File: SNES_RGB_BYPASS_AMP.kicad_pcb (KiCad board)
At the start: 2 copper layers, 16 x 29.5 mm, 16 parts, among them J1 RGB_Input, J2 SNES Multiout, U1 THS7374

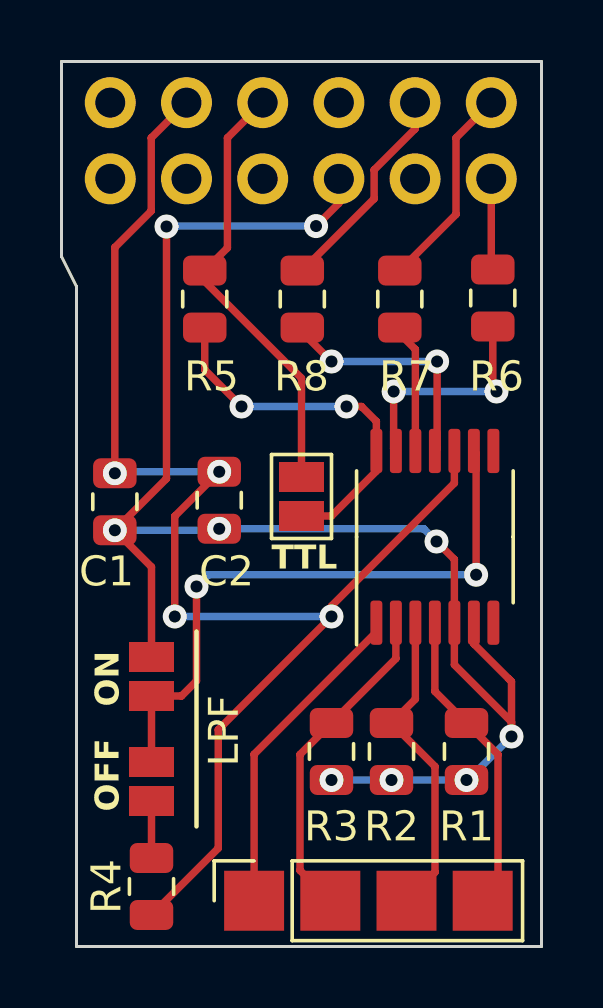
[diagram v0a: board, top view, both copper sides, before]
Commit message: Update silkscreen
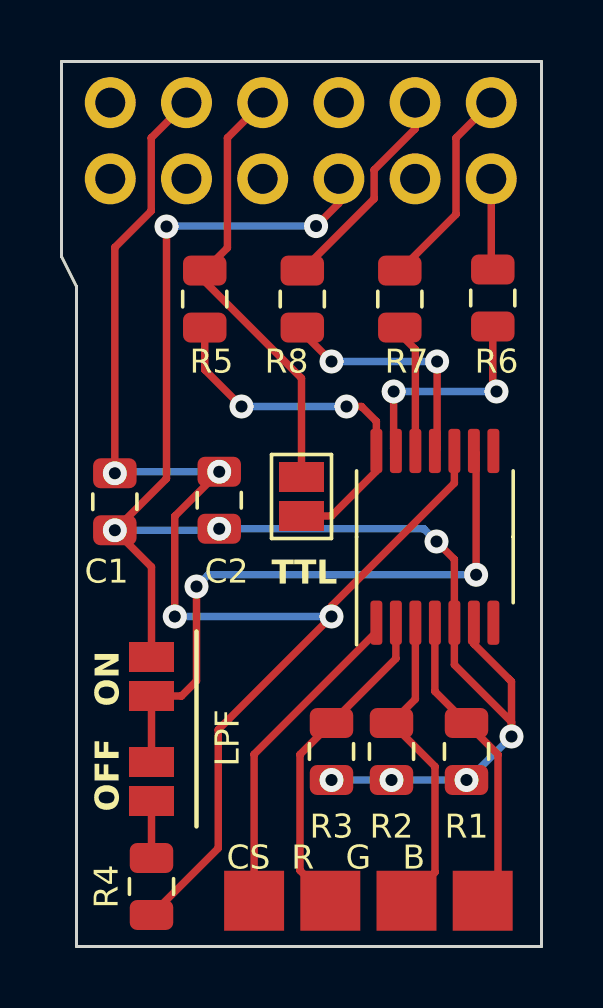
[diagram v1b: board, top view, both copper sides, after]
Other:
- board text added: "CS R G B"
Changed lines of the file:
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@@
     (property "ki_keywords" "cap capacitor")
     (attr smd)
-    (fp_text reference "C1" (at 2.3244 0.278 -180) (layer "F.SilkS")
-        (effects (font (size 1 1) (thickness 0.15)))
+    (fp_text reference "C1" (at 2.3244 0.278 180) (layer "F.SilkS")
+        (effects (font (size 0.8 0.8) (thickness 0.15)))
     )
     (fp_text value "1uF" (at 0 1.68 90) (layer "F.Fab")
@@
     (property "ki_keywords" "R res resistor")
     (attr smd)
-    (fp_text reference "R5" (at 2.5808 -0.2248 -180) (layer "F.SilkS")
-        (effects (font (size 1 1) (thickness 0.15)))
+    (fp_text reference "R5" (at 2.0808 -0.2248 180) (layer "F.SilkS")
+        (effects (font (size 0.8 0.8) (thickness 0.15)))
     )
     (fp_text value "75" (at 0 1.68 90) (layer "F.Fab")
@@
     (attr smd)
     (fp_text reference "R4" (at 0 1.5 90) (layer "F.SilkS")
-        (effects (font (size 1 1) (thickness 0.15)))
+        (effects (font (size 0.8 0.8) (thickness 0.15)))
     )
     (fp_text value "10K" (at 0 1.68 90) (layer "F.Fab")
@@
     (attr smd)
     (fp_text reference "R3" (at -2.5 0 180) (layer "F.SilkS")
-        (effects (font (size 1 1) (thickness 0.15)))
+        (effects (font (size 0.8 0.8) (thickness 0.15)))
     )
     (fp_text value "750" (at 0 1.68 90) (layer "F.Fab")
@@
         (effects (font (size 1 1) (thickness 0.15)))
     )
-    (fp_line (start -1.33 1.27) (end -1.33 8.95)
-      (stroke (width 0.12) (type solid)) (layer "F.SilkS"))
-    (fp_line (start -1.33 1.27) (end 1.33 1.27)
-      (stroke (width 0.12) (type solid)) (layer "F.SilkS"))
-    (fp_line (start -1.33 8.95) (end 1.33 8.95)
-      (stroke (width 0.12) (type solid)) (layer "F.SilkS"))
-    (fp_line (start 0 -1.33) (end 1.33 -1.33)
-      (stroke (width 0.12) (type solid)) (layer "F.SilkS"))
-    (fp_line (start 1.33 -1.33) (end 1.33 0)
-      (stroke (width 0.12) (type solid)) (layer "F.SilkS"))
-    (fp_line (start 1.33 1.27) (end 1.33 8.95)
-      (stroke (width 0.12) (type solid)) (layer "F.SilkS"))
     (fp_line (start -1.8 -1.8) (end 1.75 -1.8)
       (stroke (width 0.05) (type solid)) (layer "F.CrtYd"))
@@
     (fp_line (start 1.75 9.4) (end -1.8 9.4)
       (stroke (width 0.05) (type solid)) (layer "F.CrtYd"))
-    (fp_line (start -1.27 -1.27) (end 0.635 -1.27)
-      (stroke (width 0.1) (type solid)) (layer "F.Fab"))
-    (fp_line (start -1.27 8.89) (end -1.27 -1.27)
-      (stroke (width 0.1) (type solid)) (layer "F.Fab"))
-    (fp_line (start 0.635 -1.27) (end 1.27 -0.635)
-      (stroke (width 0.1) (type solid)) (layer "F.Fab"))
-    (fp_line (start 1.27 -0.635) (end 1.27 8.89)
-      (stroke (width 0.1) (type solid)) (layer "F.Fab"))
-    (fp_line (start 1.27 8.89) (end -1.27 8.89)
-      (stroke (width 0.1) (type solid)) (layer "F.Fab"))
     (pad "1" smd rect (at 0 0 90) (size 2 2) (layers "F.Cu" "F.Paste" "F.Mask")
       (net 3 "/CSync") (pinfunction "Pin_1") (pintype "passive"))
@@
     (attr smd)
     (fp_text reference "R2" (at -2.5 0 180) (layer "F.SilkS")
-        (effects (font (size 1 1) (thickness 0.15)))
+        (effects (font (size 0.8 0.8) (thickness 0.15)))
     )
     (fp_text value "750" (at 0 1.68 90) (layer "F.Fab")
@@
     (property "ki_keywords" "R res resistor")
     (attr smd)
-    (fp_text reference "R7" (at 2.5808 -0.2224 -180) (layer "F.SilkS")
-        (effects (font (size 1 1) (thickness 0.15)))
+    (fp_text reference "R7" (at 2.0808 -0.2224 180) (layer "F.SilkS")
+        (effects (font (size 0.8 0.8) (thickness 0.15)))
     )
     (fp_text value "75" (at 0 1.68 90) (layer "F.Fab")
@@
     (property "ki_keywords" "R res resistor")
     (attr smd)
-    (fp_text reference "R8" (at 2.5808 0.0264 -180) (layer "F.SilkS")
-        (effects (font (size 1 1) (thickness 0.15)))
+    (fp_text reference "R8" (at 2.0808 0.5264 180) (layer "F.SilkS")
+        (effects (font (size 0.8 0.8) (thickness 0.15)))
     )
     (fp_text value "75" (at 0 1.68 90) (layer "F.Fab")
@@
     (attr smd)
     (fp_text reference "R1" (at -2.5 0 180) (layer "F.SilkS")
-        (effects (font (size 1 1) (thickness 0.15)))
+        (effects (font (size 0.8 0.8) (thickness 0.15)))
     )
     (fp_text value "750" (at 0 1.68 90) (layer "F.Fab")
@@
     (property "ki_keywords" "R res resistor")
     (attr smd)
-    (fp_text reference "R6" (at 2.6164 -0.1236 -180) (layer "F.SilkS")
-        (effects (font (size 1 1) (thickness 0.15)))
+    (fp_text reference "R6" (at 2.1164 -0.1236 180) (layer "F.SilkS")
+        (effects (font (size 0.8 0.8) (thickness 0.15)))
     )
     (fp_text value "75" (at 0 1.68 90) (layer "F.Fab")
@@
     (property "ki_keywords" "cap capacitor")
     (attr smd)
-    (fp_text reference "C2" (at 2.3752 -0.2422 -180) (layer "F.SilkS")
-        (effects (font (size 1 1) (thickness 0.15)))
+    (fp_text reference "C2" (at 2.3752 -0.2422 180) (layer "F.SilkS")
+        (effects (font (size 0.8 0.8) (thickness 0.15)))
     )
     (fp_text value "0.1uF" (at 0 1.68 90) (layer "F.Fab")
@@
   (gr_line (start 127.5 77) (end 127.5 99)
     (stroke (width 0.1) (type default)) (layer "Edge.Cuts"))
-  (gr_text "TTL" (at 134 86.5) (layer "F.SilkS")
-    (effects (font (size 0.8 0.8) (thickness 0.1) bold) (justify left bottom))
+  (gr_text "CS  R   G   B" (at 132.5 96.5) (layer "F.SilkS")
+    (effects (font (size 0.8 0.8) (thickness 0.15)) (justify left bottom))
+  )
+  (gr_text "TTL" (at 134 87) (layer "F.SilkS")
+    (effects (font (size 0.8 0.8) (thickness 0.15) bold) (justify left bottom))
   )
   (gr_text "ON" (at 129 91 90) (layer "F.SilkS")
-    (effects (font (size 0.8 0.8) (thickness 0.1) bold) (justify left bottom))
+    (effects (font (size 0.8 0.8) (thickness 0.15) bold) (justify left bottom))
   )
   (gr_text "LPF" (at 133 93 90) (layer "F.SilkS")
-    (effects (font (size 1 1) (thickness 0.15)) (justify left bottom))
+    (effects (font (size 0.8 0.8) (thickness 0.15)) (justify left bottom))
   )
   (gr_text "OFF" (at 129 94.5 90) (layer "F.SilkS")
-    (effects (font (size 0.8 0.8) (thickness 0.1) bold) (justify left bottom))
+    (effects (font (size 0.8 0.8) (thickness 0.15) bold) (justify left bottom))
   )
   (segment (start 131.1656 70.871) (end 129.9906 72.046) (width 0.25) (layer "F.Cu") (net 1))
